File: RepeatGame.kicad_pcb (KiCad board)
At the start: 2 copper layers, 45 x 45 mm, 27 parts, among them J1 BATTERY, J2 AVR-ISP-6, SW1 YELLOW, SW2 BLUE, SW3 ORANGE, SW4 RED, SW5 POWER, U1 ATmega328P-AU, Y1 12MHz

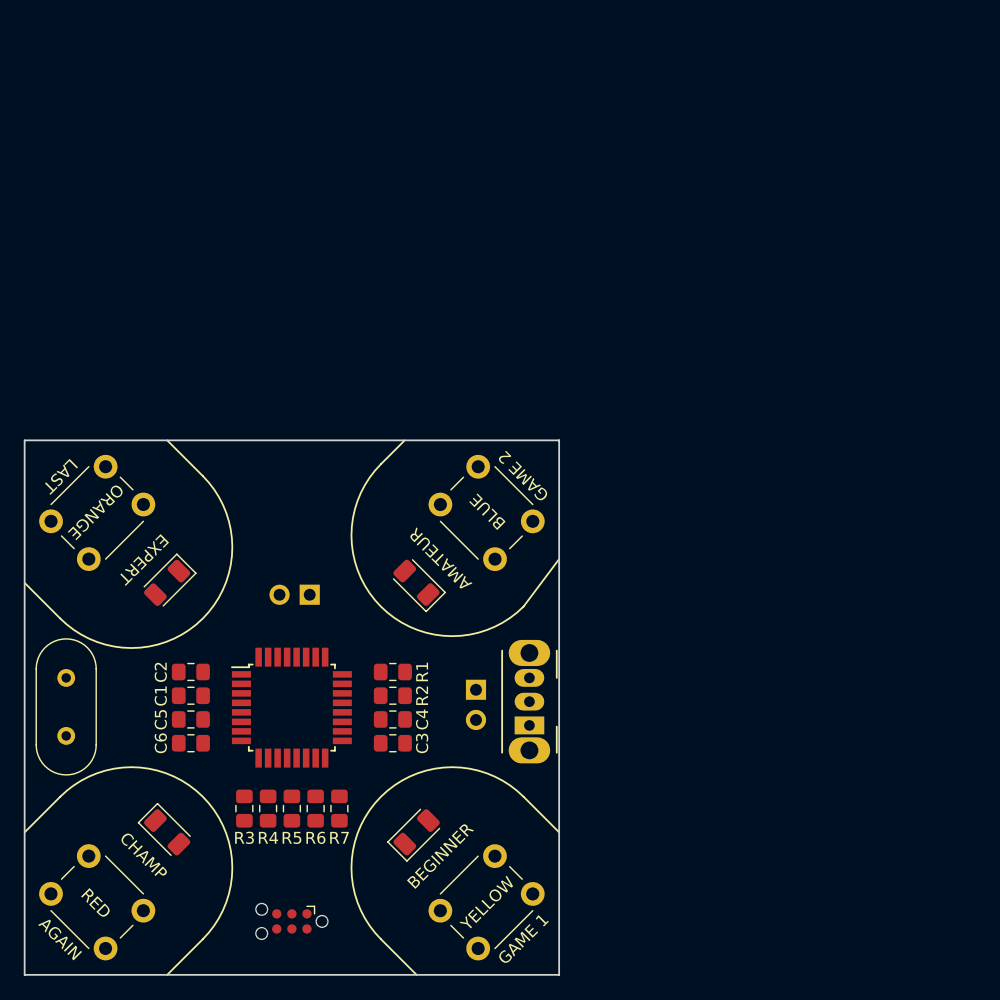
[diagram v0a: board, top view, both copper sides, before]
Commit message: Routing
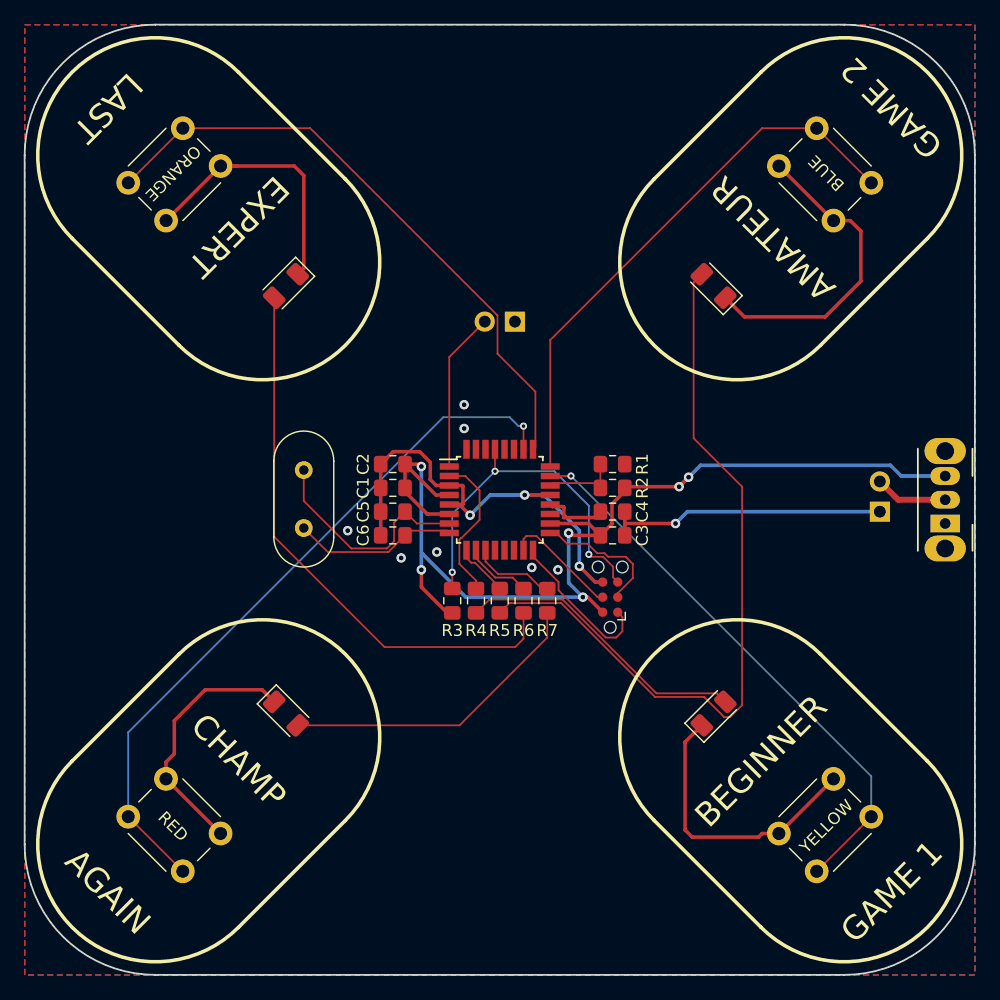
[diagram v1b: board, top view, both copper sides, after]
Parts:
- moved SW2 40.3 mm to (163.1, 46.5)
- moved SW5 38.9 mm to (172.5, 72.0)
- moved J2 38.3 mm to (144.3, 78.2), turned to 90 degrees
- moved J1 37.2 mm to (167.0, 71.0), turned to 0 degrees
- moved D2 35.4 mm to (153.0, 52.0)
- moved SW3 29.2 mm to (111.5, 41.9)
- moved SW1 29.2 mm to (158.5, 98.1)
- moved LS1 28.8 mm to (136.3, 55.0)
- moved D1 26.9 mm to (153.0, 88.0)
- moved D3 26.9 mm to (117.0, 52.0)
- moved Y1 26.6 mm to (118.5, 67.5)
- moved C3 25.5 mm to (144.5, 73.0)
- moved C4 25.5 mm to (144.5, 71.0)
- moved R1 25.5 mm to (144.5, 69.0)
- moved R2 25.5 mm to (144.5, 67.0)
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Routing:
- net GND: track 0.00 -> 159.2 mm, vias 0 -> 11
- net VCC: track 0.00 -> 91.4 mm, vias 0 -> 6
- net Net-(D2-Pad2): track 0.00 -> 63.4 mm
- net /K8: track 0.00 -> 60.1 mm, vias 0 -> 1
- net /K4: track 0.00 -> 52.2 mm
- net Net-(D3-Pad2): track 0.00 -> 47.4 mm
- net /K1: track 0.00 -> 47.4 mm, vias 0 -> 1
- net /K2: track 0.00 -> 47.0 mm
- net ~RESET: track 0.00 -> 30.3 mm, vias 0 -> 3
- net Net-(D4-Pad2): track 0.00 -> 26.1 mm
- net Net-(D1-Pad2): track 0.00 -> 25.0 mm
- net /XTAL1: track 0.00 -> 19.1 mm
- net /XTAL2: track 0.00 -> 13.9 mm
- net /BUZZER: track 0.00 -> 13.4 mm
- net MISO: track 0.00 -> 13.3 mm
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- added copper zone on B.Cu, net GND
- added copper zone on F.Cu, net GND
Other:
- board size 45 x 45 mm -> 80 x 80 mm
- net class Default: clearance 0.2 -> 0.15; trace_width 0.25 -> 0.15; via_dia 0.8 -> 0.6; via_drill 0.4 -> 0.3
- net class POWER added: clearance 0.2, trace_width 0.3, via_dia 0.8, via_drill 0.4
- net class VBATT added: clearance 0.2, trace_width 0.5, via_dia 0.8, via_drill 0.4
- rule pad_to_mask_clearance: 0.2 -> 0.1
- rule trace_clearance: 0.2 -> 0.15
- rule trace_min: 0.2 -> 0.15
- rule via_min_size: 0.4 -> 0.6
- board text added: "JLCJLCJLCJLC"
- board text added: "Repeat Game Rev A 2019 Dominic Thibodeau dev@hotkeysoft.net"

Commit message: Added source
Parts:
- R4, R6, R7: value 220 -> 330
- R5: value 100 -> 330
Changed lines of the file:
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@@
       (effects (font (size 1 1) (thickness 0.15)))
     )
-    (fp_text value 220 (at 0 1.65 90) (layer F.Fab)
+    (fp_text value 330 (at 0 1.65 90) (layer F.Fab)
       (effects (font (size 1 1) (thickness 0.15)))
     )
@@
       (effects (font (size 1 1) (thickness 0.15)))
     )
-    (fp_text value 220 (at 0 1.65 90) (layer F.Fab)
+    (fp_text value 330 (at 0 1.65 90) (layer F.Fab)
       (effects (font (size 1 1) (thickness 0.15)))
     )
@@
       (effects (font (size 1 1) (thickness 0.15)))
     )
-    (fp_text value 100 (at 0 1.65 90) (layer F.Fab)
+    (fp_text value 330 (at 0 1.65 90) (layer F.Fab)
       (effects (font (size 1 1) (thickness 0.15)))
     )
@@
       (effects (font (size 1 1) (thickness 0.15)))
     )
-    (fp_text value 220 (at 0 1.65 90) (layer F.Fab)
+    (fp_text value 330 (at 0 1.65 90) (layer F.Fab)
       (effects (font (size 1 1) (thickness 0.15)))
     )
